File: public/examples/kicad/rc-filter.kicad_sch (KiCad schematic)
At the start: 2 parts

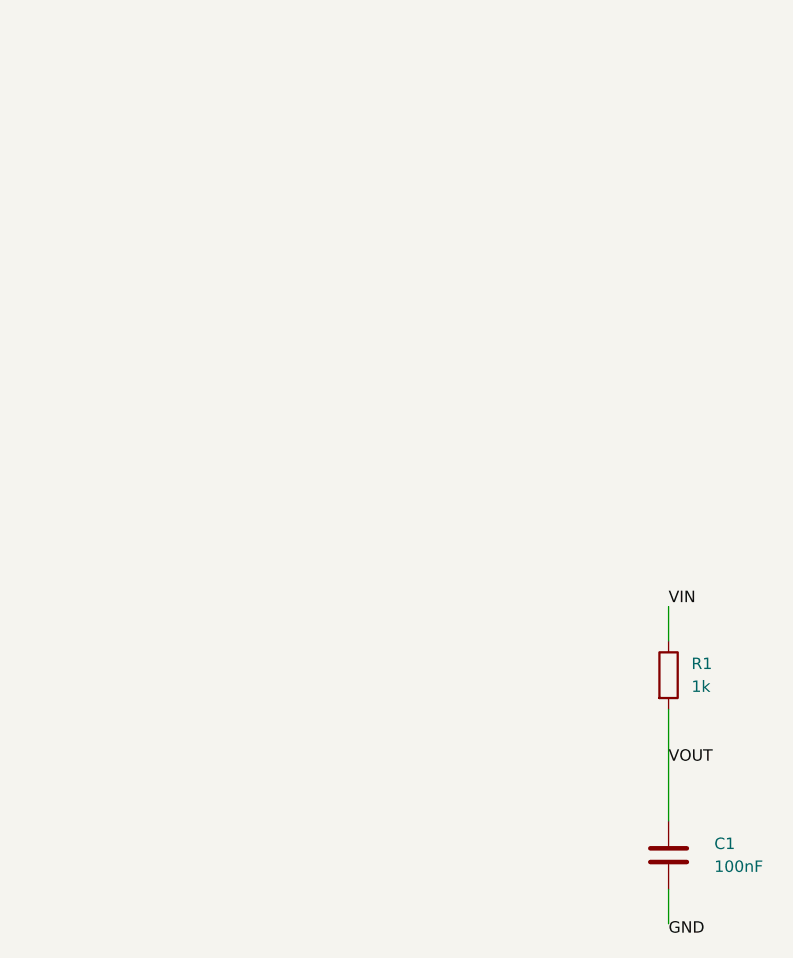
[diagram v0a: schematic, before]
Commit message: up
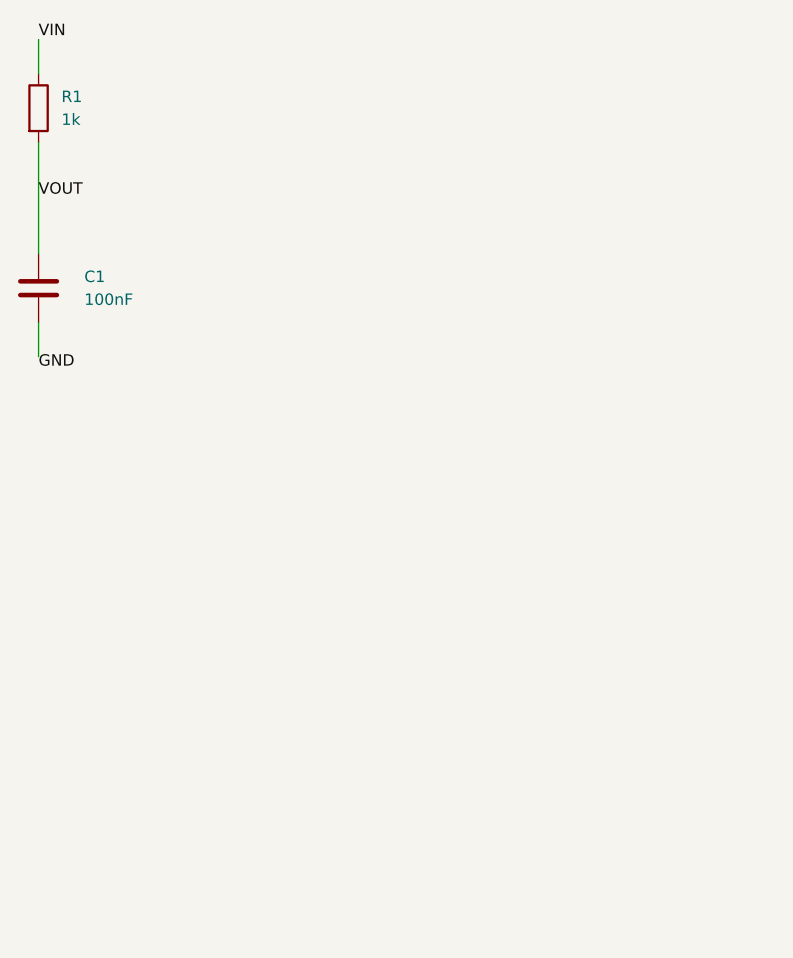
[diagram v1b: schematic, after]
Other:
- moved on the sheet: C1, R1
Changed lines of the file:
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@@
 	(generator "eeschema")
 	(generator_version "10.0")
-	(paper "A4")
+	(paper "User" 60 70)
 	(wire
 		(pts
-			(xy 100 86.19) (xy 100 82.38)
+			(xy 30 23.19) (xy 30 19.38)
 		)
 		(stroke
@@
 	(wire
 		(pts
-			(xy 100 113.81) (xy 100 117.62)
+			(xy 30 50.81) (xy 30 54.62)
 		)
 		(stroke
@@
 	(wire
 		(pts
-			(xy 100 93.81) (xy 100 106.19)
+			(xy 30 30.81) (xy 30 43.19)
 		)
 		(stroke
@@
 	)
 	(label "GND"
-		(at 100 117.62 0)
+		(at 30 54.62 0)
 		(effects
 			(font
@@
 	)
 	(label "VOUT"
-		(at 100 100 0)
+		(at 30 37 0)
 		(effects
 			(font
@@
 	)
 	(label "VIN"
-		(at 100 82.38 0)
+		(at 30 19.38 0)
 		(effects
 			(font
@@
 	(symbol
 		(lib_id "Device:R")
-		(at 100 90 0)
+		(at 30 27 0)
 		(unit 1)
 		(body_style 1)
@@
 		(fields_autoplaced yes)
 		(property "Reference" "R1"
-			(at 102.54 88.73 0)
+			(at 32.54 25.73 0)
 			(show_name no)
 			(do_not_autoplace no)
@@
 		)
 		(property "Value" "1k"
-			(at 102.54 91.27 0)
+			(at 32.54 28.27 0)
 			(show_name no)
 			(do_not_autoplace no)
@@
 	(symbol
 		(lib_id "Device:C")
-		(at 100 110 0)
+		(at 30 47 0)
 		(unit 1)
 		(body_style 1)
@@
 		(fields_autoplaced yes)
 		(property "Reference" "C1"
-			(at 105.08 108.73 0)
+			(at 35.08 45.73 0)
 			(show_name no)
 			(do_not_autoplace no)
@@
 		)
 		(property "Value" "100nF"
-			(at 105.08 111.27 0)
+			(at 35.08 48.27 0)
 			(show_name no)
 			(do_not_autoplace no)
